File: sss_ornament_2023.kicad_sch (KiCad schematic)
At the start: 38 parts, among them J1 Conn_01x02_Male, J2 Conn_01x01, J3 GND, J4 V_PIR, J5 PIR_TIME, Q1 Q_PMOS_DGS, U1 ATtiny412-SS

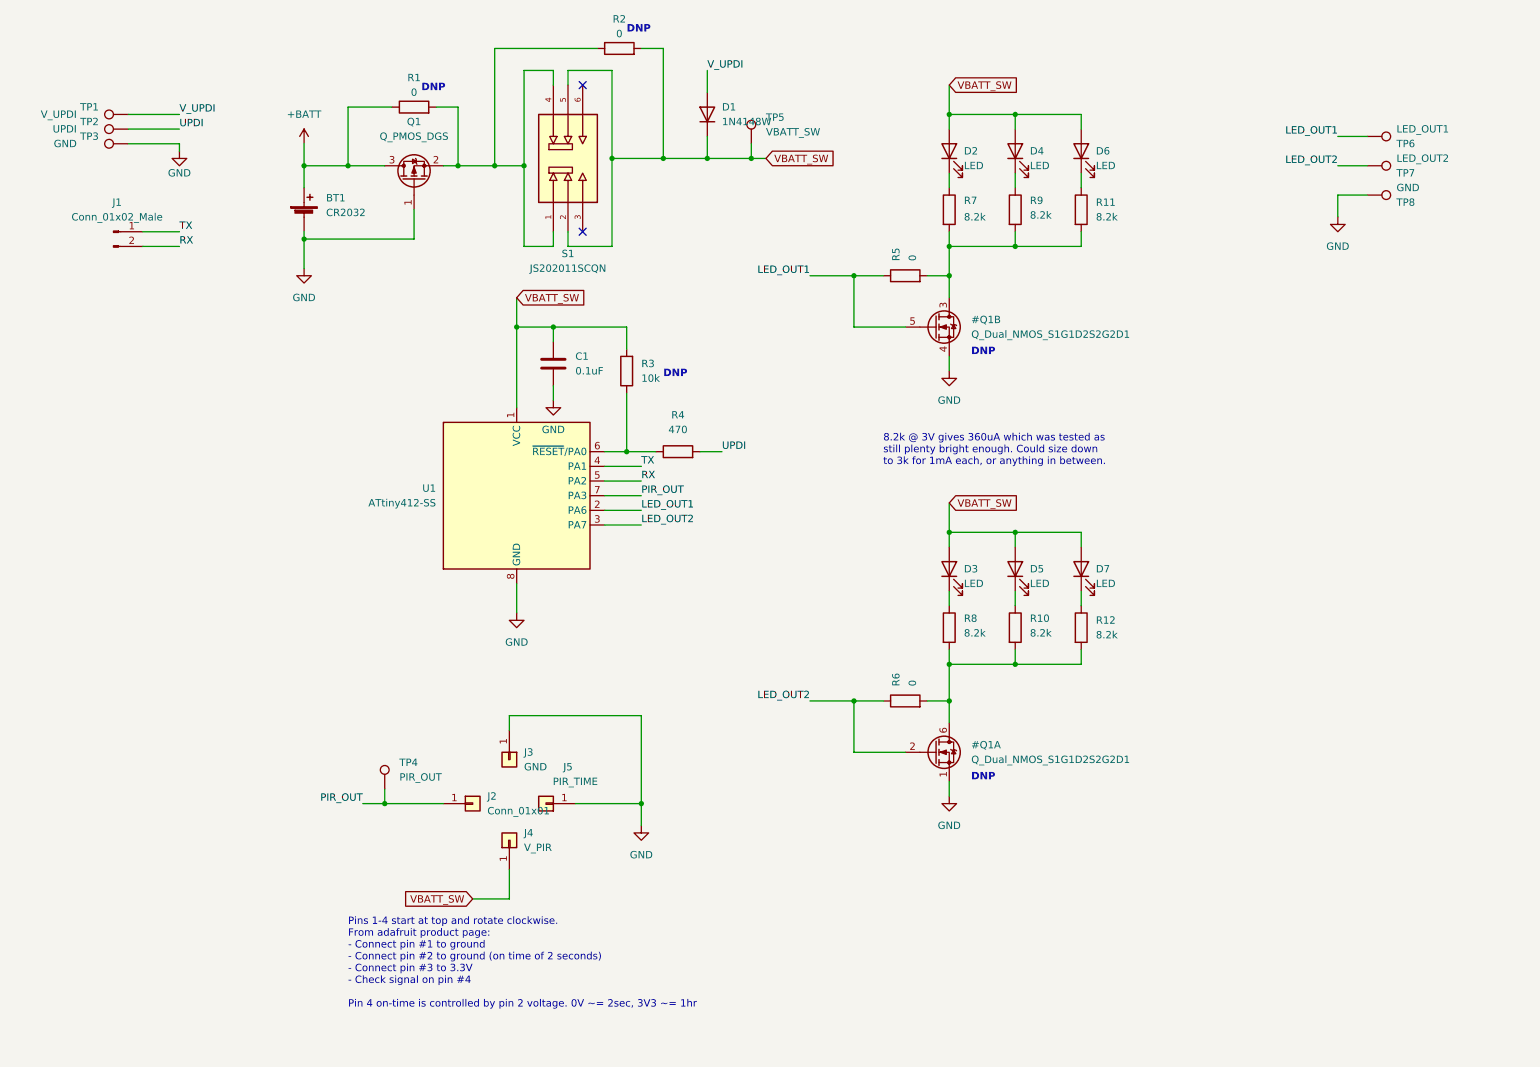
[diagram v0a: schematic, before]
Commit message: Completed 2023 ornament kicad project and all necessary bom/gerber/datasheet/document data
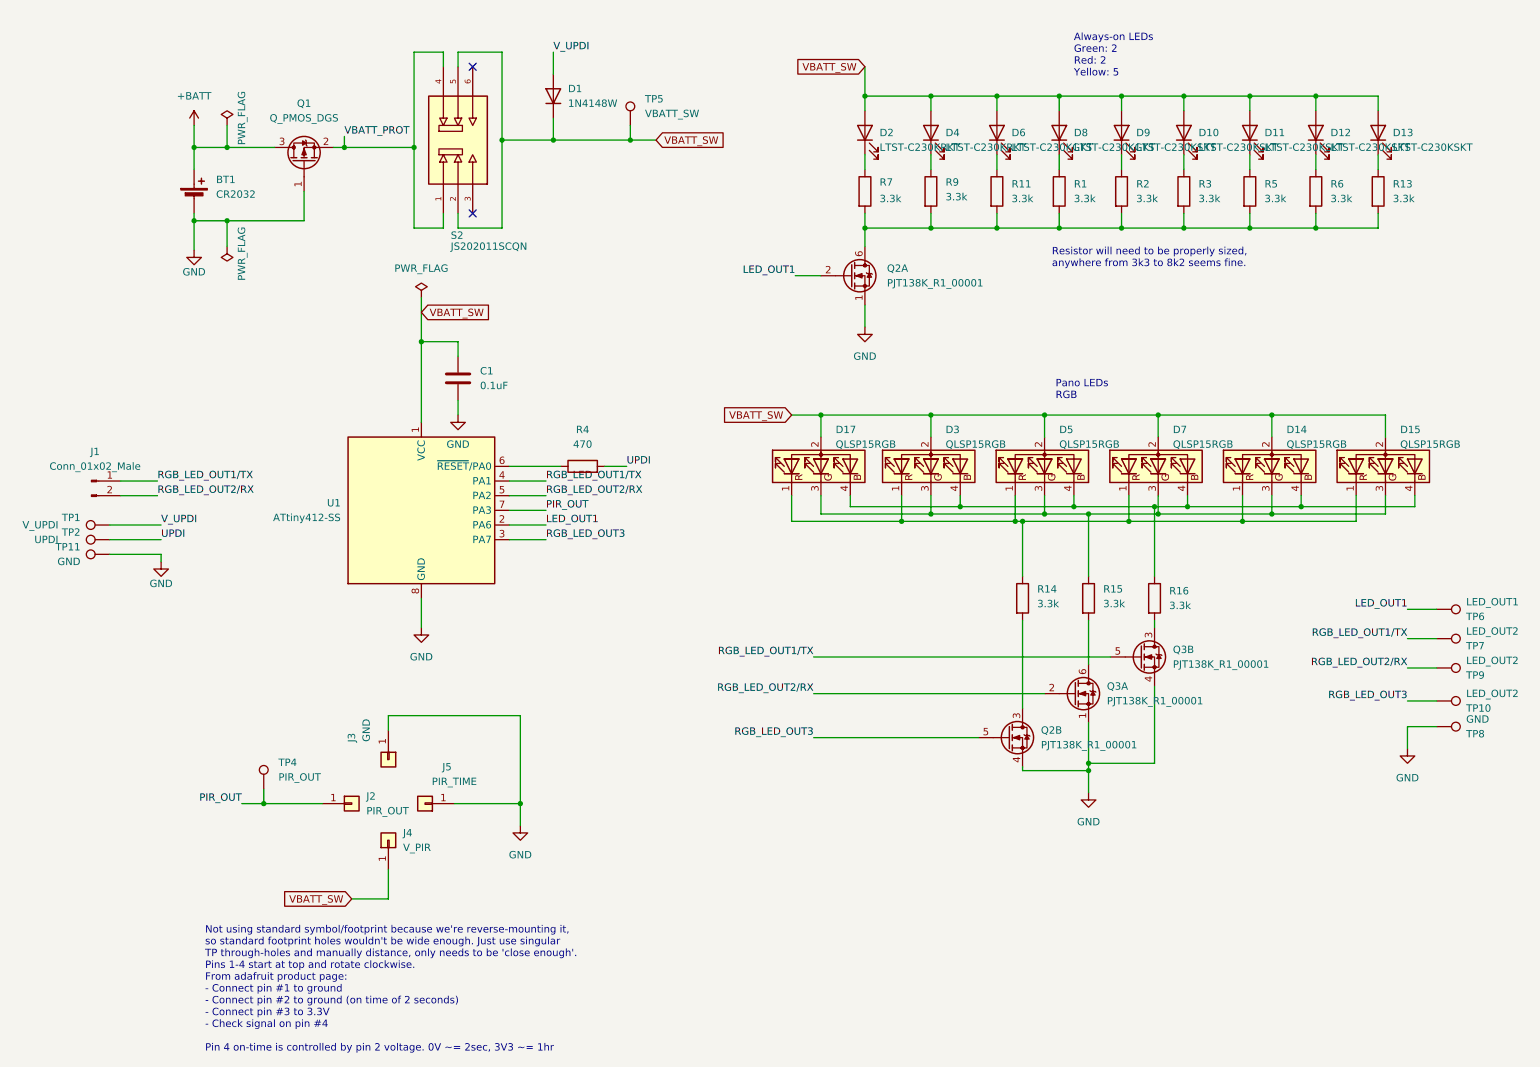
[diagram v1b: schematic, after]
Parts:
- removed #Q1: Q_Dual_NMOS_S1G1D2S2G2D1, Package_SO:SO-8_3.9x4.9mm_P1.27mm, symbol Device:Q_Dual_NMOS_S1G1D2S2G2D1
- removed D3, D5, D7: LED, LED_SMD:LED_0603_1608Metric_Pad1.05x0.95mm_HandSolder, symbol Device:LED
- removed R10, R12, R8: 8.2k, Resistor_SMD:R_0805_2012Metric_Pad1.20x1.40mm_HandSolder, symbol Device:R
- removed S1: JS202011SCQN, Custom Footprints:SW_JS202011SCQN, symbol JS202011SCQN:JS202011SCQN
- removed TP3: GND, TestPoint:TestPoint_Pad_D2.0mm, symbol Connector:TestPoint
- added D10, D11, D12, D13, D9: LTST-C230KSKT, LTST-C230K:LED_LTST-C230K, symbol Device:LED
- added D14, D15, D17, D3, D5, D7: QLSP15RGB, QLSP15RGB:QLSP15RGB, symbol Device:LED_RAGB
- added D8: LTST-C230KGKT, LTST-C230K:LED_LTST-C230K, symbol Device:LED
- added Q2, Q3: PJT138K_R1_00001, Package_TO_SOT_SMD:SOT-363_SC-70-6_Handsoldering, symbol Device:Q_Dual_NMOS_S1G1D2S2G2D1
- added R13, R14, R15, R16: 3.3k, Resistor_SMD:R_0805_2012Metric_Pad1.20x1.40mm_HandSolder, symbol Device:R
- added S2: JS202011SCQN, SW_JS202011SCQN, symbol JS202011SCQN:JS202011SCQN
- added TP10, TP9: LED_OUT2, TestPoint:TestPoint_Pad_D2.0mm, symbol Connector:TestPoint
- added TP11: GND, TestPoint:TestPoint_Pad_D2.0mm, symbol Connector:TestPoint
- BT1: footprint Battery:BatteryHolder_AdamTech_BH-67D-5_1x2032 -> Battery:BatteryHolder_Keystone_3002_1x2032
- D2, D4: value LED -> LTST-C230KRKT; footprint LED_SMD:LED_0603_1608Metric_Pad1.05x0.95mm_HandSolder -> LTST-C230K:LED_LTST-C230K
- D6: value LED -> LTST-C230KGKT; footprint LED_SMD:LED_0603_1608Metric_Pad1.05x0.95mm_HandSolder -> LTST-C230K:LED_LTST-C230K
- J1: symbol Connector:Conn_01x02_Male -> Connector:Conn_01x02_Pin
- J2: value Conn_01x01 -> PIR_OUT
- R1, R2, R5, R6: value 0 -> 3.3k
- R11, R7, R9: value 8.2k -> 3.3k
- R3: value 10k -> 3.3k
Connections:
- net +BATT: no longer R1.1
- net GND: now also Q2.1 (S), Q2.4 (S), Q3.1 (S), Q3.4 (S), TP11.1
- net LED_OUT1: now also Q2.2 (G); no longer R5.1
- net VBATT_SW: now also D10.2 (A), D11.2 (A), D12.2 (A), D13.2 (A), D14.2 (A), D15.2 (A), D17.2 (A), D3.2 (A), D5.2 (A), D7.2 (A), D8.2 (A), D9.2 (A), S2.2, S2.5; no longer R2.2, R3.2
- net at R4.1, U1.6 (~{RESET}/PA0): no longer R3.1
- net at R11.2, R5.2, R7.2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: now also R1.2, R2.2, R3.2, R6.2, Q2.6 (D), R13.2
- removed net LED_OUT2: R6.1, TP7.1, U1.3 (PA7)
- net RX renamed RGB_LED_OUT2/RX
- net RGB_LED_OUT2/RX: now also Q3.2 (G), TP9.1
- net TX renamed RGB_LED_OUT1/TX
- net RGB_LED_OUT1/TX: now also TP7.1, Q3.5 (G)
- new net: D9.1 (K), R2.1
- new net: D10.1 (K), R3.1
- new net: D13.1 (K), R13.1
- new net: D8.1 (K), R1.1
- new net: D14.3 (GK), D15.3 (GK), D17.3 (GK), D3.3 (GK), D5.3 (GK), D7.3 (GK), R15.1
- new net: Q3.6 (D), R15.2
- new net: D14.1 (RK), D15.1 (RK), D17.1 (RK), D3.1 (RK), D5.1 (RK), D7.1 (RK), R14.1
- new net: D14.4 (BK), D15.4 (BK), D17.4 (BK), D3.4 (BK), D5.4 (BK), D7.4 (BK), R16.1
- new net: Q2.3 (D), R14.2
- new net: D11.1 (K), R5.1
- new net: Q3.3 (D), R16.2
- new net: D12.1 (K), R6.1
- new net RGB_LED_OUT3: Q2.5 (G), TP10.1, U1.3 (PA7)
- new net VBATT_PROT: Q1.2 (S), S2.1, S2.4
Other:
- note added: "Always-on LEDs Green: 2 Red: 2 Yellow: 5"
- note added: "Not using standard symbol/footprint because we're reverse-mounting it, so standard footprint holes wouldn't be wide enough. Just use singular TP through-holes and manually distance, only needs to be 'close enough'. Pins 1-4 start at top and rotate clockwise. From adafruit product page: - Connect pin #1 to ground - Connect pin #2 to ground (on time of 2 seconds) - Connect pin #3 to 3.3V - Check si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"
- note added: "Pano LEDs RGB"
- note added: "Resistor will need to be properly sized, anywhere from 3k3 to 8k2 seems fine."
- note removed: "8.2k @ 3V gives 360uA which was tested as still plenty bright enough. Could size down to 3k for 1mA each, or anything in between."
- note removed: "DNP"
- note removed: "Pins 1-4 start at top and rotate clockwise. From adafruit product page: - Connect pin #1 to ground - Connect pin #2 to ground (on time of 2 seconds) - Connect pin #3 to 3.3V - Check signal on pin #4 Pin 4 on-time is controlled by pin 2 voltage. 0V ~= 2sec, 3V3 ~= 1hr"
- moved on the sheet: BT1, C1, D1, D2, D4, D6, J1, J2, J4, J5, Q1, R11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
